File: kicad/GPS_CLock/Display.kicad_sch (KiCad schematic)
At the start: 7 parts, among them J501 1-1734839-6

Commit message: updated pcb
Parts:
- C501, C504: footprint (none) -> Capacitor_SMD:C_0402_1005Metric
- R501, R502: footprint (none) -> Resistor_SMD:R_0402_1005Metric
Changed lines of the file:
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@@
       (effects (font (size 1.27 1.27)) (justify right))
     )
-    (property "Footprint" "" (id 2) (at 146.05 105.41 0)
+    (property "Footprint" "Capacitor_SMD:C_0402_1005Metric" (id 2) (at 146.05 105.41 0)
       (effects (font (size 1.27 1.27)) hide)
     )
@@
       (effects (font (size 1.27 1.27)) (justify right))
     )
-    (property "Footprint" "" (id 2) (at 153.67 106.68 0)
+    (property "Footprint" "Capacitor_SMD:C_0402_1005Metric" (id 2) (at 153.67 106.68 0)
       (effects (font (size 1.27 1.27)) hide)
     )
@@
       (effects (font (size 1.27 1.27)) (justify right))
     )
-    (property "Footprint" "" (id 2) (at 138.43 104.14 0)
+    (property "Footprint" "Resistor_SMD:R_0402_1005Metric" (id 2) (at 138.43 104.14 0)
       (effects (font (size 1.27 1.27)) hide)
     )
@@
       (effects (font (size 1.27 1.27)) (justify right))
     )
-    (property "Footprint" "" (id 2) (at 140.97 91.44 0)
+    (property "Footprint" "Resistor_SMD:R_0402_1005Metric" (id 2) (at 140.97 91.44 0)
       (effects (font (size 1.27 1.27)) hide)
     )

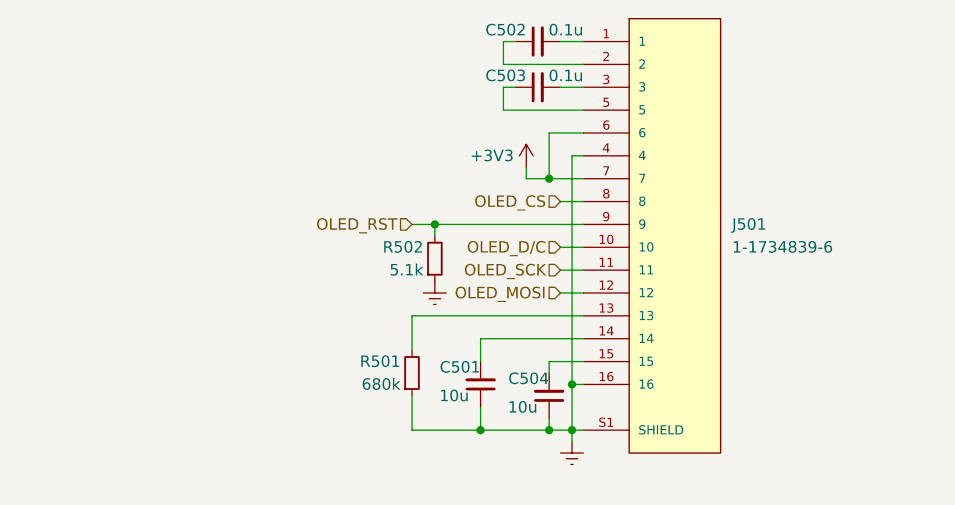
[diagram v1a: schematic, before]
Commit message: update pcb
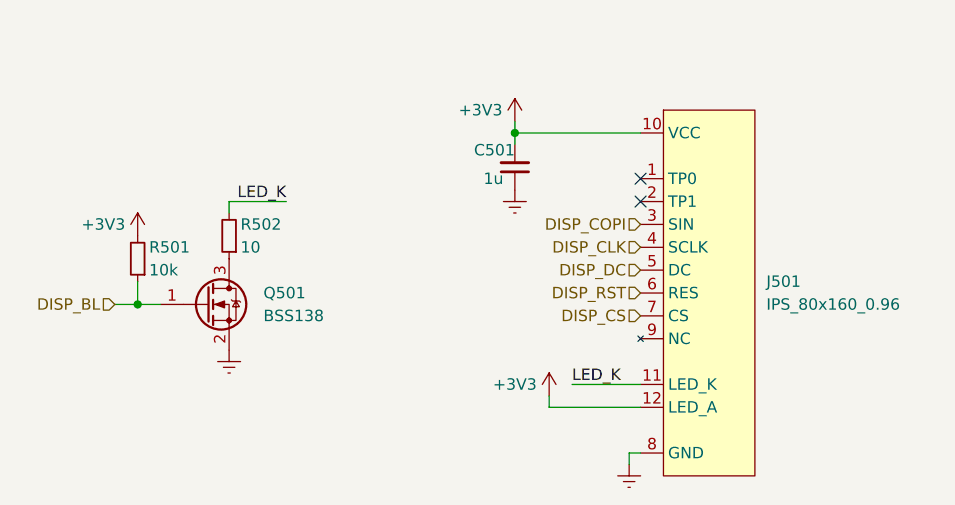
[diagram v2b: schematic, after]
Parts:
- removed C501: 10u, Capacitor_SMD:C_0402_1005Metric, symbol Device:C_Small
- removed C502, C503: 0.1u, Capacitor_SMD:C_0402_1005Metric, symbol Device:C_Small
- removed J501: 1-1734839-6, clock:TE_1-1734839-6, symbol Clock:1-1734839-6
- removed R501: 680k, Resistor_SMD:R_0402_1005Metric, symbol Device:R_Small
- added J501: IPS_80x160_0.96, clock:IPS_FPC-13, symbol Clock:IPS_80x160_0.96
- added Q501: BSS138, Package_TO_SOT_SMD:SOT-23, symbol Transistor_FET:BSS138
- added R502: 10, Resistor_SMD:R_0402_1005Metric, symbol Device:R_Small
- C501: renamed from C504; value 10u -> 1u
- R501: renamed from R502; value 5.1k -> 10k
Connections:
- net OLED_RST is gone; now on net +3V3: R501.2
- net +3V3: now also C501.2, J501.10 (VCC), J501.12 (LED_A)
- net Earth: now also J501.13 (GND), J501.8 (GND), Q501.2 (S); no longer R501.1
- new net: Q501.3 (D), R502.1
- new net DISP_BL: Q501.1 (G), R501.1
- new net DISP_CLK: J501.4 (SCLK)
- new net DISP_COPI: J501.3 (SIN)
- new net DISP_CS: J501.7 (CS)
- new net DISP_DC: J501.5 (DC)
- new net DISP_RST: J501.6 (RES)
- new net LED_K: J501.11 (LED_K), R502.2
- no-connect marks 0 -> 2
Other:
- moved on the sheet: C501, R501
